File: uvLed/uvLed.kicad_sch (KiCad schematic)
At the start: 5 parts, among them J1 Conn_01x02

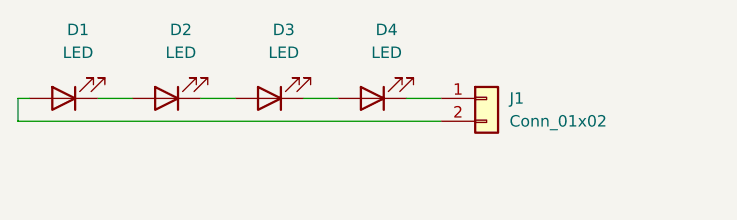
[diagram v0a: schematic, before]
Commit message: schematic
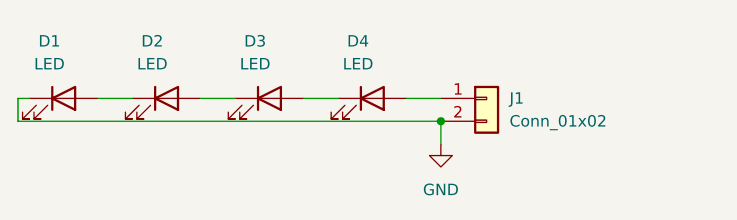
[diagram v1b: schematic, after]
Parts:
- D1, D2, D3, D4: footprint (none) -> uvLED:SMD-2
- J1: footprint (none) -> Connector_PinHeader_2.54mm:PinHeader_1x02_P2.54mm_Vertical
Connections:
- net at D2.1 (K): now also D1.2 (A); no longer D3.2 (A)
- net at D2.2 (A): now also D3.1 (K); no longer D1.1 (K)
- net at D4.1 (K): now also D3.2 (A); no longer J1.1 (Pin_1)
- net at D4.2 (A): now also J1.1 (Pin_1); no longer D3.1 (K)
- net GND: now reaches J1.2 (Pin_2)
- net GND: now also D1.1 (K); no longer D1.2 (A)
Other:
- moved on the sheet: D1, D2, D3, D4
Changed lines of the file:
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@@
 (kicad_sch (version 20230121) (generator eeschema)
   (paper "A4")
+  (junction (at 167.64 91.44) (diameter 0) (color 0 0 0 0)
+  )
   (wire (pts (xy 120.65 91.44) (xy 120.65 88.9))
     (stroke (width 0) (type default))
@@
     (stroke (width 0) (type default))
   )
+  (wire (pts (xy 167.64 91.44) (xy 167.64 93.98))
+    (stroke (width 0) (type default))
+  )
   (wire (pts (xy 167.64 91.44) (xy 120.65 91.44))
     (stroke (width 0) (type default))
   )
-  (symbol (lib_id "Device:LED") (at 137.16 88.9 180) (unit 1)
+  (symbol (lib_id "Device:LED") (at 137.16 88.9 0) (unit 1)
     (in_bom yes) (on_board yes) (dnp no) (fields_autoplaced)
-    (property "Reference" "D2" (at 138.7475 81.28 0)
+    (property "Reference" "D2" (at 135.5725 82.55 0)
       (effects (font (size 1.27 1.27)))
     )
-    (property "Value" "LED" (at 138.7475 83.82 0)
+    (property "Value" "LED" (at 135.5725 85.09 0)
       (effects (font (size 1.27 1.27)))
     )
-    (property "Footprint" "" (at 137.16 88.9 0)
+    (property "Footprint" "uvLED:SMD-2" (at 137.16 88.9 0)
       (effects (font (size 1.27 1.27)) hide)
     )
@@
     )
   )
-  (symbol (lib_id "Device:LED") (at 160.02 88.9 180) (unit 1)
+  (symbol (lib_id "Device:LED") (at 160.02 88.9 0) (unit 1)
     (in_bom yes) (on_board yes) (dnp no) (fields_autoplaced)
-    (property "Reference" "D4" (at 161.6075 81.28 0)
+    (property "Reference" "D4" (at 158.4325 82.55 0)
       (effects (font (size 1.27 1.27)))
     )
-    (property "Value" "LED" (at 161.6075 83.82 0)
+    (property "Value" "LED" (at 158.4325 85.09 0)
       (effects (font (size 1.27 1.27)))
     )
-    (property "Footprint" "" (at 160.02 88.9 0)
+    (property "Footprint" "uvLED:SMD-2" (at 160.02 88.9 0)
       (effects (font (size 1.27 1.27)) hide)
     )
@@
     )
   )
-  (symbol (lib_id "Device:LED") (at 125.73 88.9 180) (unit 1)
+  (symbol (lib_id "power:GND") (at 167.64 93.98 0) (unit 1)
     (in_bom yes) (on_board yes) (dnp no) (fields_autoplaced)
-    (property "Reference" "D1" (at 127.3175 81.28 0)
+    (property "Reference" "#PWR01" (at 167.64 100.33 0)
+      (effects (font (size 1.27 1.27)) hide)
+    )
+    (property "Value" "GND" (at 167.64 99.06 0)
       (effects (font (size 1.27 1.27)))
     )
-    (property "Value" "LED" (at 127.3175 83.82 0)
+    (property "Footprint" "" (at 167.64 93.98 0)
+      (effects (font (size 1.27 1.27)) hide)
+    )
+    (property "Datasheet" "" (at 167.64 93.98 0)
+      (effects (font (size 1.27 1.27)) hide)
+    )
+    (pin "1")
+    (instances
+      (project "uvLed"
+        (path "/b3a6664e-4928-48cf-b65b-34c0a168bb21"
+          (reference "#PWR01") (unit 1)
+        )
+      )
+    )
+  )
+  (symbol (lib_id "Device:LED") (at 125.73 88.9 0) (unit 1)
+    (in_bom yes) (on_board yes) (dnp no) (fields_autoplaced)
+    (property "Reference" "D1" (at 124.1425 82.55 0)
       (effects (font (size 1.27 1.27)))
     )
-    (property "Footprint" "" (at 125.73 88.9 0)
+    (property "Value" "LED" (at 124.1425 85.09 0)
+      (effects (font (size 1.27 1.27)))
+    )
+    (property "Footprint" "uvLED:SMD-2" (at 125.73 88.9 0)
       (effects (font (size 1.27 1.27)) hide)
     )
@@
     )
   )
-  (symbol (lib_id "Device:LED") (at 148.59 88.9 180) (unit 1)
+  (symbol (lib_id "Device:LED") (at 148.59 88.9 0) (unit 1)
     (in_bom yes) (on_board yes) (dnp no) (fields_autoplaced)
-    (property "Reference" "D3" (at 150.1775 81.28 0)
+    (property "Reference" "D3" (at 147.0025 82.55 0)
       (effects (font (size 1.27 1.27)))
     )
-    (property "Value" "LED" (at 150.1775 83.82 0)
+    (property "Value" "LED" (at 147.0025 85.09 0)
       (effects (font (size 1.27 1.27)))
     )
-    (property "Footprint" "" (at 148.59 88.9 0)
+    (property "Footprint" "uvLED:SMD-2" (at 148.59 88.9 0)
       (effects (font (size 1.27 1.27)) hide)
     )
@@
       (effects (font (size 1.27 1.27)) (justify left))
     )
-    (property "Footprint" "" (at 172.72 88.9 0)
+    (property "Footprint" "Connector_PinHeader_2.54mm:PinHeader_1x02_P2.54mm_Vertical" (at 172.72 88.9 0)
       (effects (font (size 1.27 1.27)) hide)
     )

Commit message: insert C
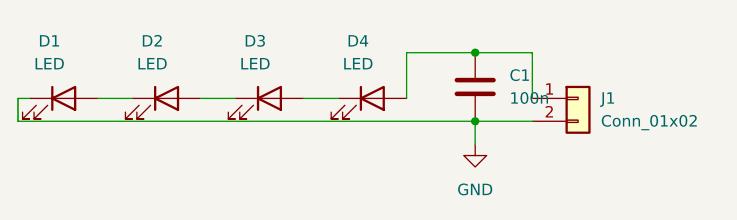
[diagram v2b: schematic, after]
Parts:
- added C1: 100n, Capacitor_SMD:C_0805_2012Metric_Pad1.18x1.45mm_HandSolder, symbol Device:C
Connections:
- net GND: now also C1.2
- net at D4.2 (A), J1.1 (Pin_1): now also C1.1
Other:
- moved on the sheet: J1
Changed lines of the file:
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@@
 (kicad_sch (version 20230121) (generator eeschema)
   (paper "A4")
-  (junction (at 167.64 91.44) (diameter 0) (color 0 0 0 0)
+  (junction (at 171.45 83.82) (diameter 0) (color 0 0 0 0)
+  )
+  (junction (at 171.45 91.44) (diameter 0) (color 0 0 0 0)
+  )
+  (wire (pts (xy 171.45 83.82) (xy 163.83 83.82))
+    (stroke (width 0) (type default))
+  )
+  (wire (pts (xy 177.8 83.82) (xy 171.45 83.82))
+    (stroke (width 0) (type default))
   )
   (wire (pts (xy 120.65 91.44) (xy 120.65 88.9))
@@
     (stroke (width 0) (type default))
   )
-  (wire (pts (xy 163.83 88.9) (xy 167.64 88.9))
+  (wire (pts (xy 177.8 88.9) (xy 177.8 83.82))
     (stroke (width 0) (type default))
   )
@@
     (stroke (width 0) (type default))
   )
+  (wire (pts (xy 163.83 83.82) (xy 163.83 88.9))
+    (stroke (width 0) (type default))
+  )
   (wire (pts (xy 129.54 88.9) (xy 133.35 88.9))
     (stroke (width 0) (type default))
   )
-  (wire (pts (xy 167.64 91.44) (xy 167.64 93.98))
+  (wire (pts (xy 171.45 91.44) (xy 177.8 91.44))
     (stroke (width 0) (type default))
   )
-  (wire (pts (xy 167.64 91.44) (xy 120.65 91.44))
+  (wire (pts (xy 171.45 91.44) (xy 171.45 93.98))
+    (stroke (width 0) (type default))
+  )
+  (wire (pts (xy 120.65 91.44) (xy 171.45 91.44))
     (stroke (width 0) (type default))
   )
@@
     )
   )
-  (symbol (lib_id "power:GND") (at 167.64 93.98 0) (unit 1)
+  (symbol (lib_id "power:GND") (at 171.45 93.98 0) (unit 1)
     (in_bom yes) (on_board yes) (dnp no) (fields_autoplaced)
-    (property "Reference" "#PWR01" (at 167.64 100.33 0)
+    (property "Reference" "#PWR01" (at 171.45 100.33 0)
       (effects (font (size 1.27 1.27)) hide)
     )
-    (property "Value" "GND" (at 167.64 99.06 0)
+    (property "Value" "GND" (at 171.45 99.06 0)
       (effects (font (size 1.27 1.27)))
     )
-    (property "Footprint" "" (at 167.64 93.98 0)
+    (property "Footprint" "" (at 171.45 93.98 0)
       (effects (font (size 1.27 1.27)) hide)
     )
-    (property "Datasheet" "" (at 167.64 93.98 0)
+    (property "Datasheet" "" (at 171.45 93.98 0)
       (effects (font (size 1.27 1.27)) hide)
     )
@@
     )
   )
-  (symbol (lib_id "Connector_Generic:Conn_01x02") (at 172.72 88.9 0) (unit 1)
+  (symbol (lib_id "Device:C") (at 171.45 87.63 0) (unit 1)
     (in_bom yes) (on_board yes) (dnp no) (fields_autoplaced)
-    (property "Reference" "J1" (at 175.26 88.9 0)
+    (property "Reference" "C1" (at 175.26 86.36 0)
       (effects (font (size 1.27 1.27)) (justify left))
     )
-    (property "Value" "Conn_01x02" (at 175.26 91.44 0)
+    (property "Value" "100n" (at 175.26 88.9 0)
       (effects (font (size 1.27 1.27)) (justify left))
     )
-    (property "Footprint" "Connector_PinHeader_2.54mm:PinHeader_1x02_P2.54mm_Vertical" (at 172.72 88.9 0)
+    (property "Footprint" "Capacitor_SMD:C_0805_2012Metric_Pad1.18x1.45mm_HandSolder" (at 172.4152 91.44 0)
       (effects (font (size 1.27 1.27)) hide)
     )
-    (property "Datasheet" "~" (at 172.72 88.9 0)
+    (property "Datasheet" "~" (at 171.45 87.63 0)
       (effects (font (size 1.27 1.27)) hide)
     )
+    (pin "2")
+    (pin "1")
+    (instances
+      (project "uvLed"
+        (path "/b3a6664e-4928-48cf-b65b-34c0a168bb21"
+          (reference "C1") (unit 1)
+        )
+      )
+    )
+  )
+  (symbol (lib_id "Connector_Generic:Conn_01x02") (at 182.88 88.9 0) (unit 1)
+    (in_bom yes) (on_board yes) (dnp no) (fields_autoplaced)
+    (property "Reference" "J1" (at 185.42 88.9 0)
+      (effects (font (size 1.27 1.27)) (justify left))
+    )
+    (property "Value" "Conn_01x02" (at 185.42 91.44 0)
+      (effects (font (size 1.27 1.27)) (justify left))
+    )
+    (property "Footprint" "Connector_PinHeader_2.54mm:PinHeader_1x02_P2.54mm_Vertical" (at 182.88 88.9 0)
+      (effects (font (size 1.27 1.27)) hide)
+    )
+    (property "Datasheet" "~" (at 182.88 88.9 0)
+      (effects (font (size 1.27 1.27)) hide)
+    )
